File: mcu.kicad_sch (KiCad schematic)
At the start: 12 parts

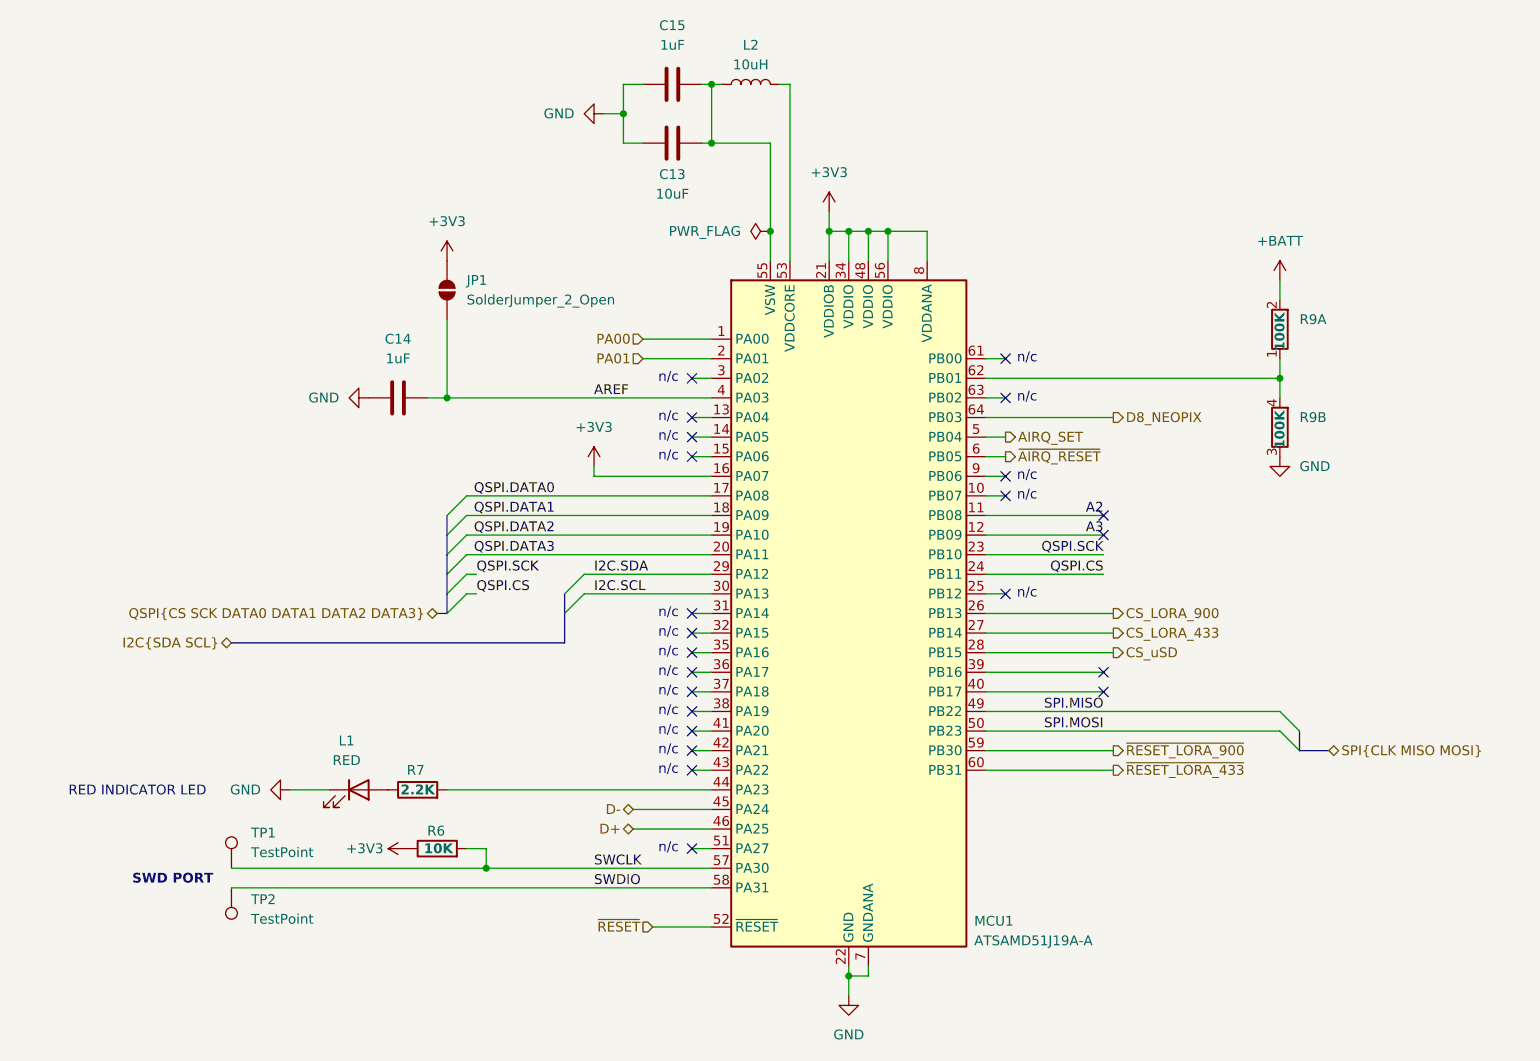
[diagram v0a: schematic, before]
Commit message: Starting layout
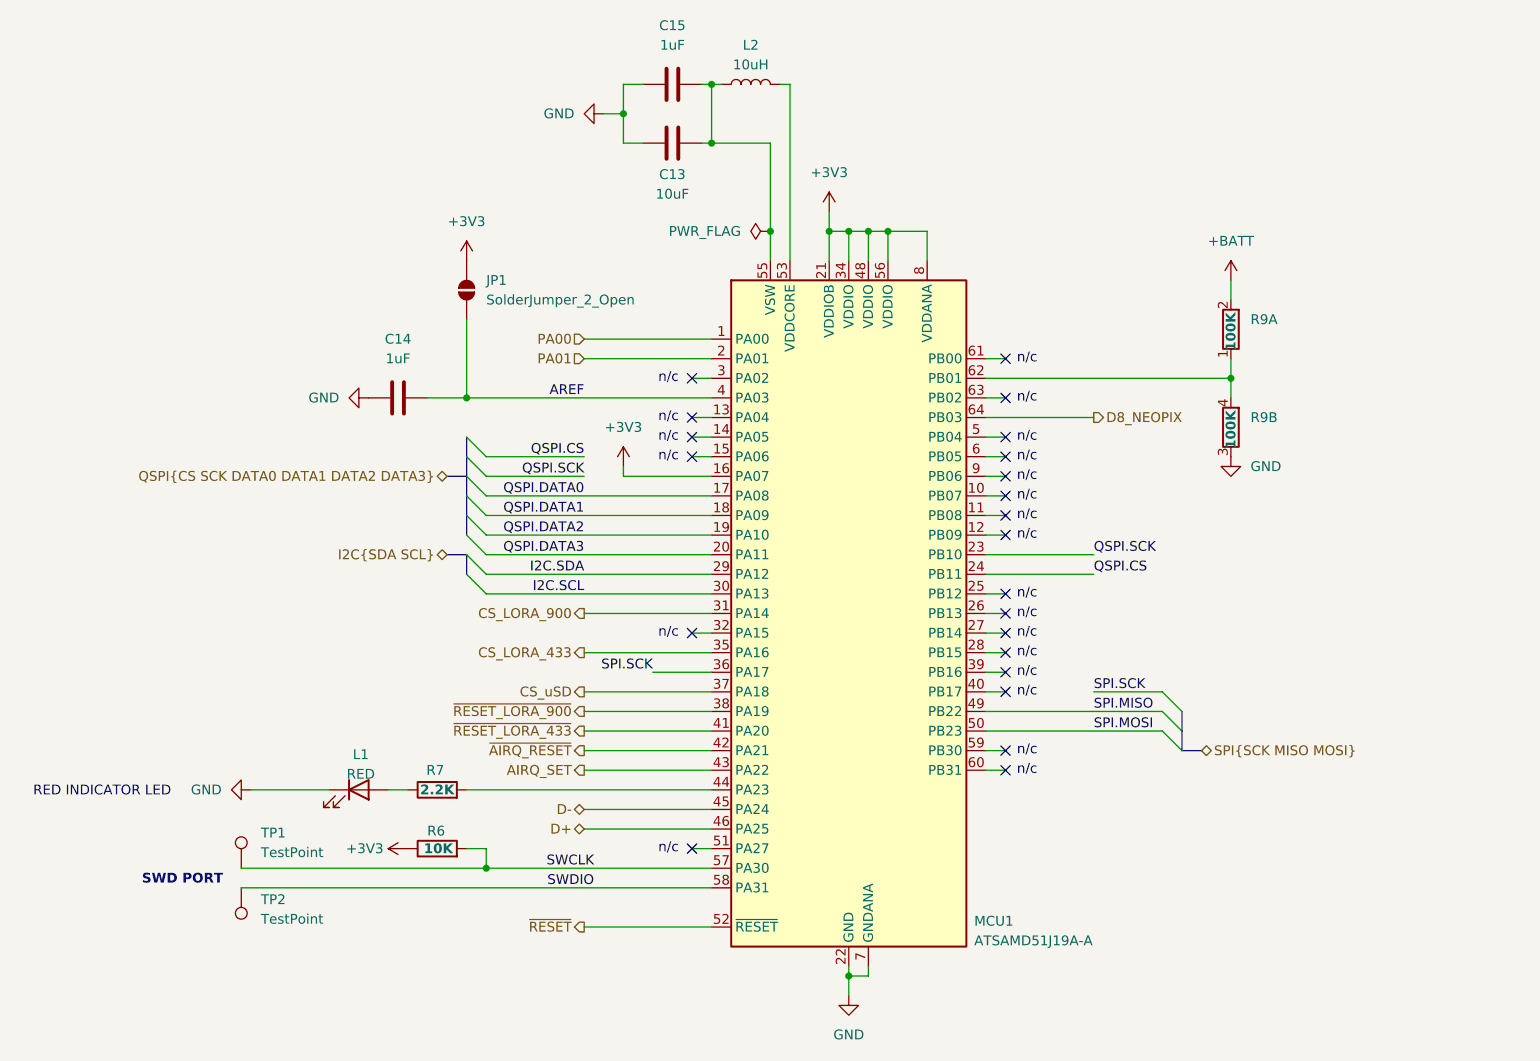
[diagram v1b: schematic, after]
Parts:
- R9: footprint Resistor_THT:R_Array_SIP8 -> Resistor_SMD:R_Array_Convex_4x1206
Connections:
- net AIRQ_SET: now also MCU1.43 (PA22); no longer MCU1.5 (PB04)
- net CS_LORA_433: now also MCU1.35 (PA16); no longer MCU1.27 (PB14)
- net CS_LORA_900: now also MCU1.31 (PA14); no longer MCU1.26 (PB13)
- net CS_uSD: now also MCU1.37 (PA18); no longer MCU1.28 (PB15)
- net ~{AIRQ_RESET}: now also MCU1.42 (PA21); no longer MCU1.6 (PB05)
- net ~{RESET_LORA_433}: now also MCU1.41 (PA20); no longer MCU1.60 (PB31)
- net ~{RESET_LORA_900}: now also MCU1.38 (PA19); no longer MCU1.59 (PB30)
- net SPI.SCK: now reaches MCU1.36 (PA17)
- net A2: no longer names the net of MCU1.11 (PB08)
- net A3: no longer names the net of MCU1.12 (PB09)
- no-connect marks 23 -> 22
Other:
- moved on the sheet: JP1, R7, R9A, R9B, TP1, TP2
